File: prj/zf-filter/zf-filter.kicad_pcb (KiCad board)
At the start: 2 copper layers, 172 x 60 mm, 66 parts

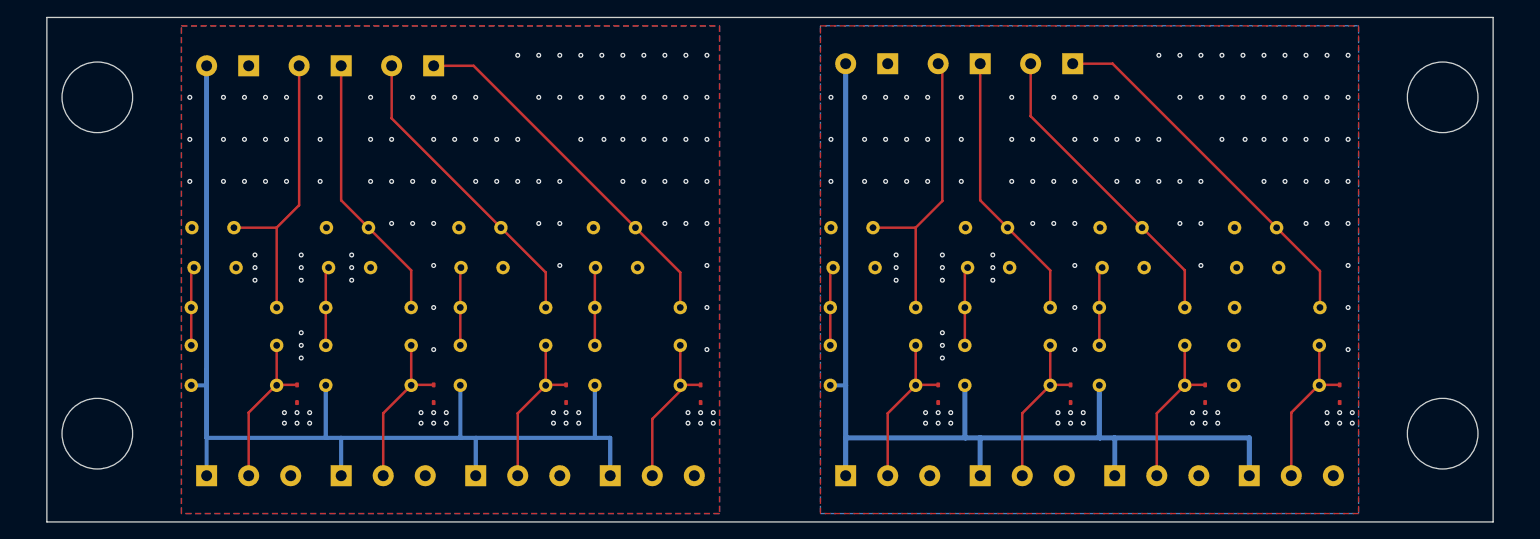
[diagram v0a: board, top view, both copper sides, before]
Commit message: zf-filter r1.0
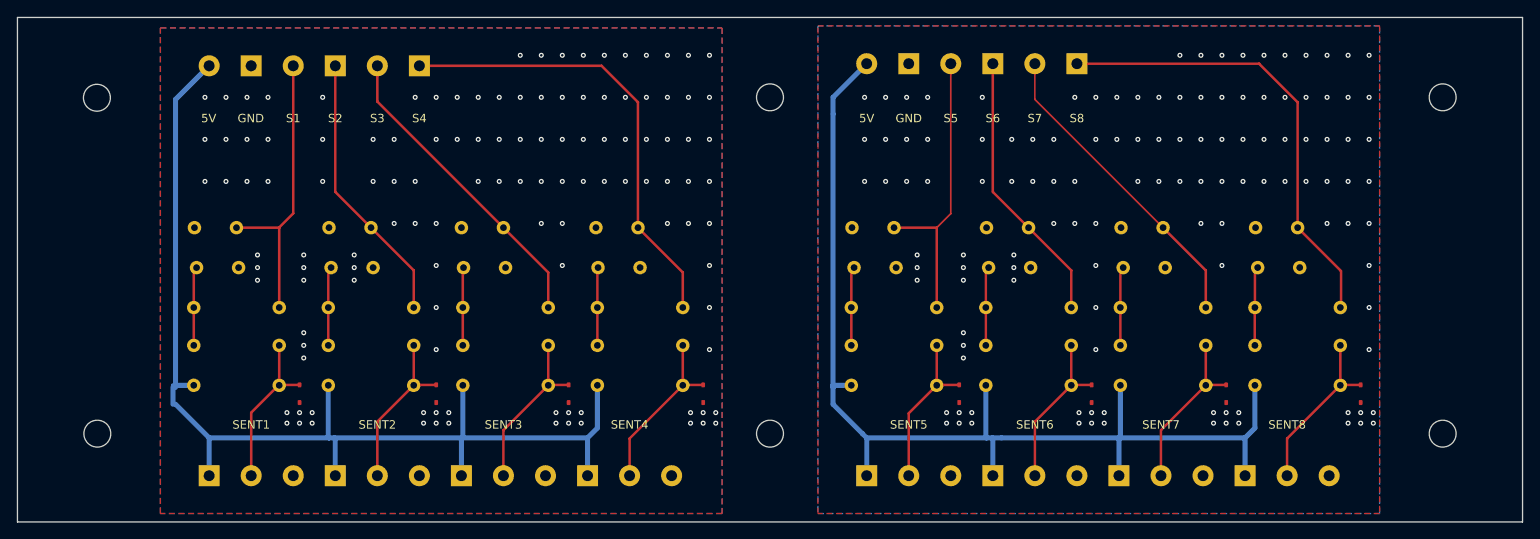
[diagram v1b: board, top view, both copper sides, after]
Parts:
- removed the REF** at (230.0, 85.0)
- removed the REF** at (70.0, 125.0)
- removed the REF** at (70.0, 85.0)
- removed the REF** at (230.0, 125.0)
- added REF**: MountingHole_3.2mm_M3, MountingHole:MountingHole_3.2mm_M3, F.Cu at (70.0, 85.0)
- added REF**: MountingHole_3.2mm_M3, MountingHole:MountingHole_3.2mm_M3, F.Cu at (150.0, 85.0)
- added REF**: MountingHole_3.2mm_M3, MountingHole:MountingHole_3.2mm_M3, F.Cu at (230.0, 85.0)
- added REF**: MountingHole_3.2mm_M3, MountingHole:MountingHole_3.2mm_M3, F.Cu at (230.0, 125.0)
- added REF**: MountingHole_3.2mm_M3, MountingHole:MountingHole_3.2mm_M3, F.Cu at (70.0, 125.0)
- added REF**: MountingHole_3.2mm_M3, MountingHole:MountingHole_3.2mm_M3, F.Cu at (150.0, 125.0)
- moved SENT4 2.70 mm to (128.3, 130.0)
- moved C51 2.50 mm to (164.8, 100.5)
- moved C52 2.50 mm to (160.0, 105.2)
- moved C61 2.50 mm to (180.8, 100.5)
- moved C62 2.50 mm to (176.0, 105.2)
- moved C71 2.50 mm to (196.8, 100.5)
- moved C72 2.50 mm to (192.0, 105.2)
- moved C81 2.50 mm to (212.8, 100.5)
- moved C82 2.50 mm to (208.0, 105.2)
- moved D50 2.50 mm to (172.5, 120.2)
- moved D60 2.50 mm to (188.2, 120.2)
- moved D70 2.50 mm to (204.2, 120.2)
- moved D80 2.50 mm to (220.2, 120.2)
- moved JP4 2.50 mm to (166.5, 81.0)
- moved R51 2.50 mm to (159.7, 114.5)
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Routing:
- net 5Va: track 176.9 -> 132.3 mm
- net S4b: track 44.0 -> 54.7 mm
- net S4a: track 43.7 -> 54.4 mm
- net Net-(C82-Pad1): track 0.00 -> 9.79 mm
- net 5Vb: track 124.9 -> 132.5 mm
- net Net-(D40-A1): track 19.3 -> 21.2 mm
- net Net-(D80-A1): track 19.4 -> 20.6 mm
- net S1b: track 35.7 -> 34.8 mm
- net S3b: track 36.6 -> 37.4 mm
- net Net-(D70-A1): track 19.3 -> 20.1 mm
- net S3a: track 36.3 -> 37.2 mm
- net Net-(D30-A1): track 19.4 -> 20.2 mm
- net GND: vias 242 -> 246
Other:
- board size 172 x 60 mm -> 179 x 60 mm
- board text added: "5V"
- board text added: "GND"
- board text added: "S1"
- board text added: "S2"
- board text added: "S3"
- board text added: "S4"
- board text added: "S5"
- board text added: "S6"
- board text added: "S7"
- board text added: "S8"
- board text removed: "${REFERENCE}"
